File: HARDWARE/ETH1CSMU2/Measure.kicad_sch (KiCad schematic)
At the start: 106 parts, among them U401 LT1790BCS6-2.5, U402 DG444DY+, U403 REF5040ID, U404 DG444DY+, U405 ADR435ARM, U406 DG419DY, U407 DG419DY, U408 DG419DY, U409 OPA141AID, U410 OPA141AID, U411 DG419DY, U412 DG419DY, U413 OPA141AID, U414 OPA141AID, U415 ADS8681IRUMT, U416 ADS8681IRUMT, U417 AD7980ARM, U418 AD7980ARM, U419 TPS76925

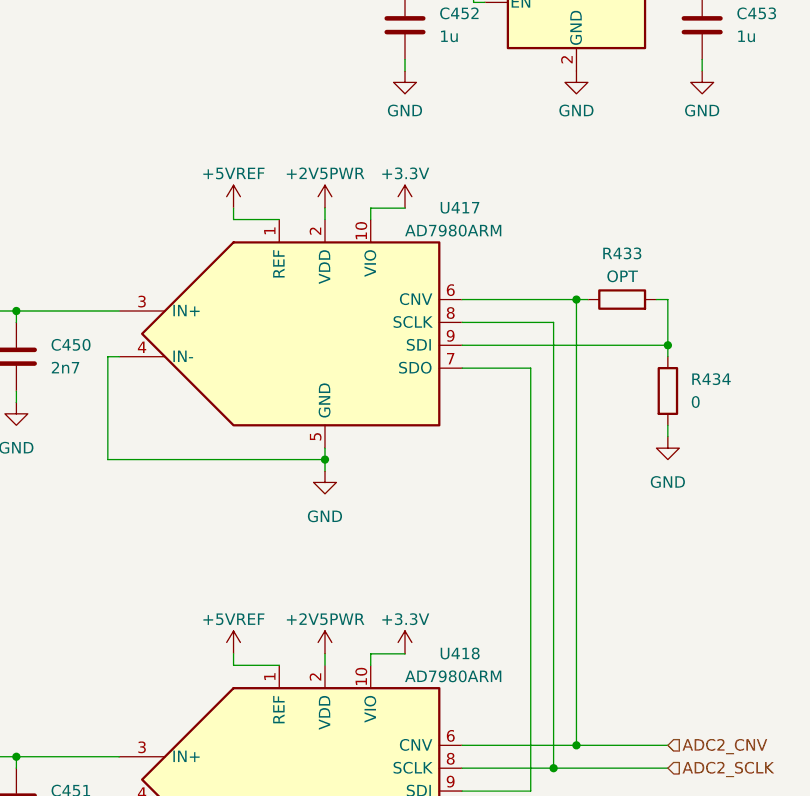
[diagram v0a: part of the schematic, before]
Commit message: PCB layout
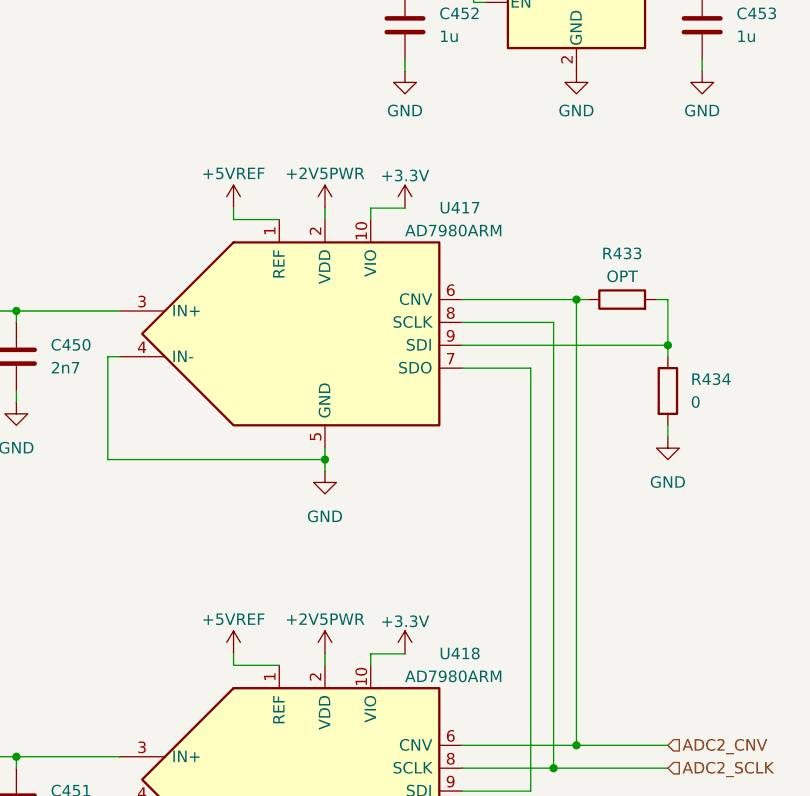
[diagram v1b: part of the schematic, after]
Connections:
- net +3V3 is gone; now on net +3.3V: U417.10 (VIO), U418.10 (VIO)
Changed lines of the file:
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@@
     (stroke (width 0) (type default) (color 0 0 0 0))
   )
-  (wire (pts (xy 170.18 115.57) (xy 172.72 115.57))
+  (wire (pts (xy 360.68 144.78) (xy 360.68 146.05))
     (stroke (width 0) (type default) (color 0 0 0 0))
   )
-  (wire (pts (xy 38.1 187.96) (xy 44.45 187.96))
+  (wire (pts (xy 170.18 115.57) (xy 172.72 115.57))
     (stroke (width 0) (type default) (color 0 0 0 0))
   )
-  (wire (pts (xy 360.68 194.31) (xy 360.68 195.58))
+  (wire (pts (xy 38.1 187.96) (xy 44.45 187.96))
     (stroke (width 0) (type default) (color 0 0 0 0))
   )
@@
     (stroke (width 0) (type default) (color 0 0 0 0))
   )
-  (wire (pts (xy 360.68 144.78) (xy 360.68 146.05))
-    (stroke (width 0) (type default) (color 0 0 0 0))
-  )
   (wire (pts (xy 119.38 251.46) (xy 107.95 251.46))
     (stroke (width 0) (type default) (color 0 0 0 0))
@@
     (stroke (width 0) (type default) (color 0 0 0 0))
   )
-  (wire (pts (xy 364.49 144.78) (xy 360.68 144.78))
-    (stroke (width 0) (type default) (color 0 0 0 0))
-  )
   (wire (pts (xy 44.45 187.96) (xy 44.45 189.23))
     (stroke (width 0) (type default) (color 0 0 0 0))
@@
     (stroke (width 0) (type default) (color 0 0 0 0))
   )
+  (wire (pts (xy 364.49 194.31) (xy 360.68 194.31))
+    (stroke (width 0) (type default) (color 0 0 0 0))
+  )
   (wire (pts (xy 198.12 123.19) (xy 201.93 123.19))
     (stroke (width 0) (type default) (color 0 0 0 0))
@@
     (stroke (width 0) (type default) (color 0 0 0 0))
   )
+  (wire (pts (xy 364.49 144.78) (xy 360.68 144.78))
+    (stroke (width 0) (type default) (color 0 0 0 0))
+  )
   (wire (pts (xy 355.6 171.45) (xy 355.6 172.72))
     (stroke (width 0) (type default) (color 0 0 0 0))
@@
     (stroke (width 0) (type default) (color 0 0 0 0))
   )
+  (wire (pts (xy 360.68 194.31) (xy 360.68 195.58))
+    (stroke (width 0) (type default) (color 0 0 0 0))
+  )
   (wire (pts (xy 36.83 100.33) (xy 36.83 102.87))
     (stroke (width 0) (type default) (color 0 0 0 0))
@@
     (stroke (width 0) (type default) (color 0 0 0 0))
   )
-  (wire (pts (xy 364.49 194.31) (xy 360.68 194.31))
-    (stroke (width 0) (type default) (color 0 0 0 0))
-  )
   (wire (pts (xy 303.53 87.63) (xy 304.8 87.63))
     (stroke (width 0) (type default) (color 0 0 0 0))
@@
     (pin "2")
   )
-  (symbol (lib_name "+3.3V_1") (lib_id "power:+3.3V") (at 364.49 194.31 0) (unit 1)
-    (in_bom yes) (on_board yes)
-    (property "Reference" "#PWR0492" (id 0) (at 364.49 198.12 0)
-      (effects (font (size 1.27 1.27)) hide)
-    )
-    (property "Value" "+3.3V" (id 1) (at 364.49 190.5 0))
-    (property "Footprint" "" (id 2) (at 364.49 194.31 0)
-      (effects (font (size 1.27 1.27)) hide)
-    )
-    (property "Datasheet" "" (id 3) (at 364.49 194.31 0)
-      (effects (font (size 1.27 1.27)) hide)
-    )
-    (pin "1")
-  )
   (symbol (lib_id "Device:C") (at 96.52 270.51 0) (unit 1)
     (in_bom yes) (on_board yes) (fields_autoplaced)
@@
     (pin "2")
   )
+  (symbol (lib_id "power:+3.3V") (at 364.49 144.78 0) (unit 1)
+    (in_bom yes) (on_board yes) (fields_autoplaced)
+    (property "Reference" "#PWR0102" (id 0) (at 364.49 148.59 0)
+      (effects (font (size 1.27 1.27)) hide)
+    )
+    (property "Value" "+3.3V" (id 1) (at 364.49 141.2042 0))
+    (property "Footprint" "" (id 2) (at 364.49 144.78 0)
+      (effects (font (size 1.27 1.27)) hide)
+    )
+    (property "Datasheet" "" (id 3) (at 364.49 144.78 0)
+      (effects (font (size 1.27 1.27)) hide)
+    )
+    (pin "1")
+  )
   (symbol (lib_id "Device:R") (at 284.48 146.05 90) (unit 1)
     (in_bom yes) (on_board yes)
@@
     (pin "1")
   )
-  (symbol (lib_name "+3.3V_1") (lib_id "power:+3.3V") (at 364.49 144.78 0) (unit 1)
-    (in_bom yes) (on_board yes)
-    (property "Reference" "#PWR0491" (id 0) (at 364.49 148.59 0)
-      (effects (font (size 1.27 1.27)) hide)
-    )
-    (property "Value" "+3.3V" (id 1) (at 364.49 140.97 0))
-    (property "Footprint" "" (id 2) (at 364.49 144.78 0)
-      (effects (font (size 1.27 1.27)) hide)
-    )
-    (property "Datasheet" "" (id 3) (at 364.49 144.78 0)
-      (effects (font (size 1.27 1.27)) hide)
-    )
-    (pin "1")
-  )
   (symbol (lib_id "power:+5V") (at 372.11 116.84 0) (unit 1)
     (in_bom yes) (on_board yes)
@@
       (effects (font (size 1.27 1.27)) hide)
     )
+    (pin "1")
+  )
+  (symbol (lib_id "power:+3.3V") (at 364.49 194.31 0) (unit 1)
+    (in_bom yes) (on_board yes) (fields_autoplaced)
+    (property "Reference" "#PWR0101" (id 0) (at 364.49 198.12 0)
+      (effects (font (size 1.27 1.27)) hide)
+    )
+    (property "Value" "+3.3V" (id 1) (at 364.49 190.7342 0))
+    (property "Footprint" "" (id 2) (at 364.49 194.31 0)
+      (effects (font (size 1.27 1.27)) hide)
+    )
+    (property "Datasheet" "" (id 3) (at 364.49 194.31 0)
+      (effects (font (size 1.27 1.27)) hide)
+    )
